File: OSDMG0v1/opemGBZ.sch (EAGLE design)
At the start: 46 parts, among them IC1 TP4056, J1 SJ2-35954D-SMT-TR, SW0 WIREPADSMD1,27-254, SW1 WIREPADSMD1,27-254, U1 FS8205, U2 FS312F-G, U3 MT3608

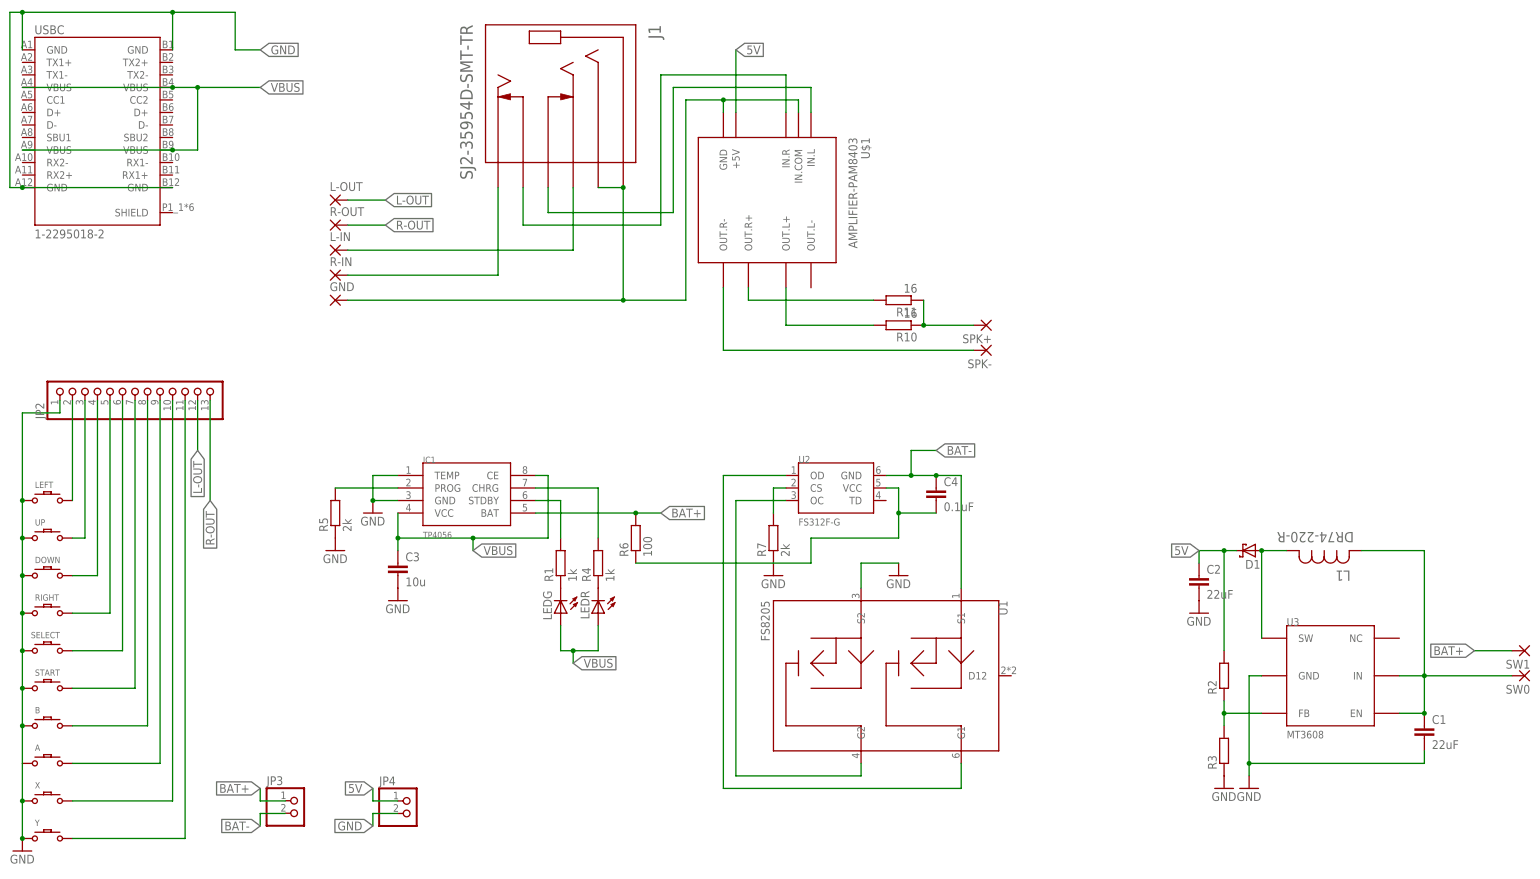
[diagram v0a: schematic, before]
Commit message: Eagle finished
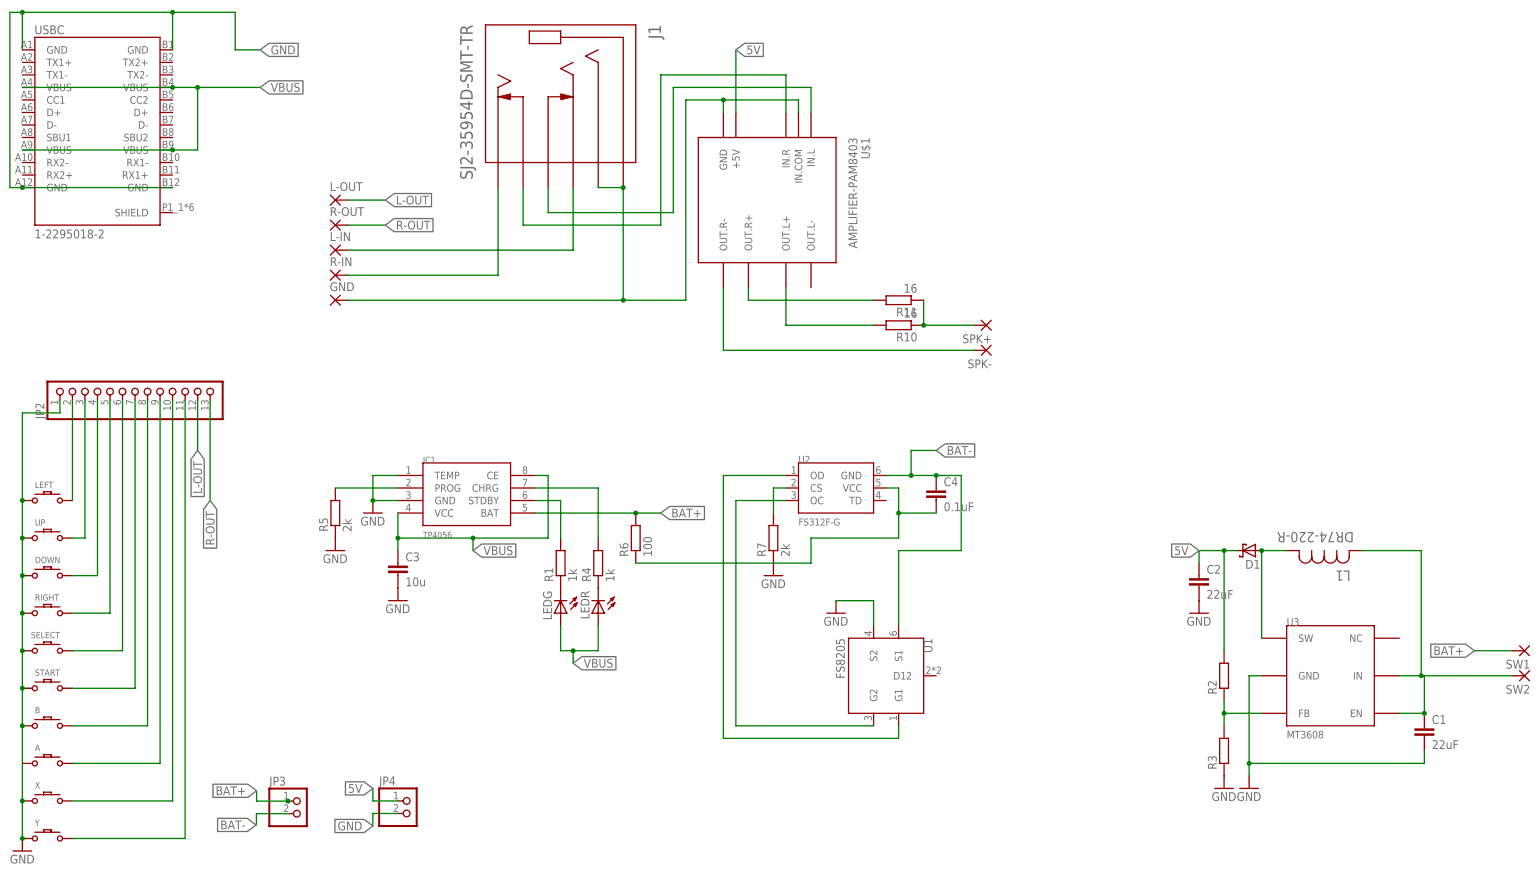
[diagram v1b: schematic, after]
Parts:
- renumbered SW0 to SW2
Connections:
- removed net L-OUT1: SW2.P
- new net N$31: C1.1, L1.2, SW2.P, U3.EN, U3.IN
- net BAT+: now also JP3.1; no longer C1.1, L1.2, U3.EN, U3.IN
- net BAT-: now also JP3.2
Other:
- moved on the sheet: JP3
